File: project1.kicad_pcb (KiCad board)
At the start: 2 copper layers, 150.4 x 48.8 mm, 53 parts, among them P1 CONN_01X02, P10 CONN_02X01, P11 CONN_02X01, P12 CONN_02X01, P13 CONN_02X01, P14 CONN_02X01, P15 CONN_02X01, P16 CONN_02X01, P17 CONN_02X01, P18 CONN_02X01, P19 CONN_02X01, P2 CONN_01X04, P20 CONN_02X01, P21 CONN_02X01, P22 CONN_02X01, P23 CONN_02X01, P24 CONN_02X01, P25 CONN_02X01, P26 CONN_02X01, P27 CONN_02X01, P28 CONN_02X01, P29 CONN_02X01, P3 CONN_02X04, P4 CONN_02X04, P5 CONN_01X04, P6 CONN_02X04, P7 CONN_02X01, P8 CONN_02X01, P9 CONN_02X01, U1 LT1460GIZ-5, U2 TS912IN

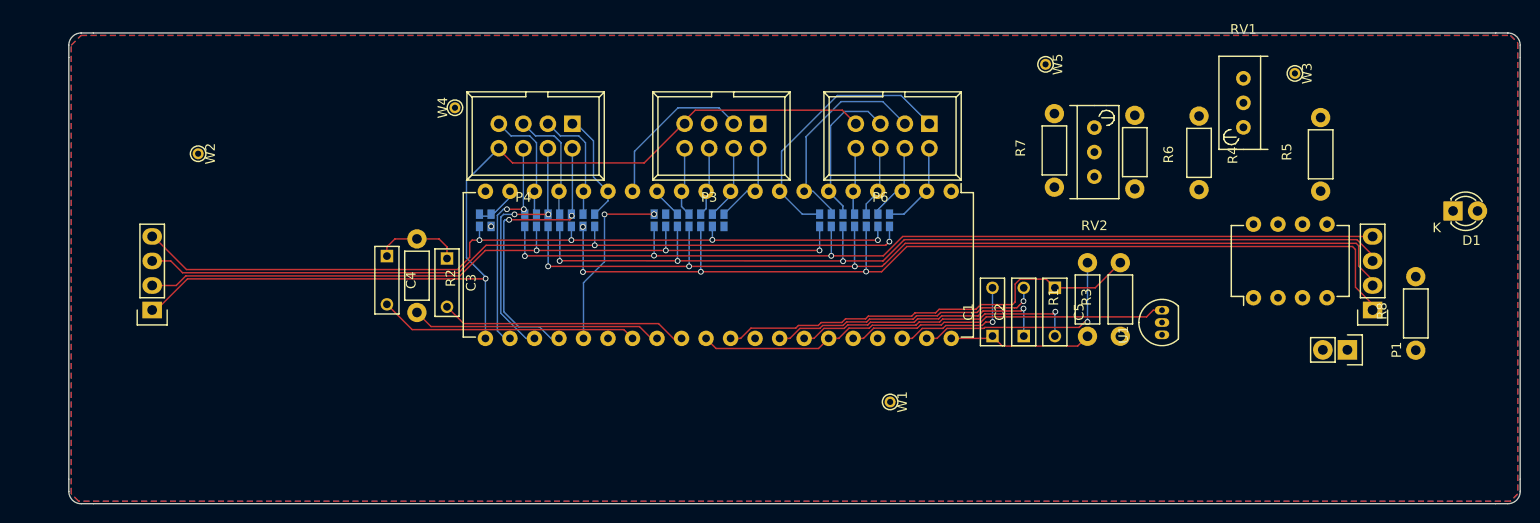
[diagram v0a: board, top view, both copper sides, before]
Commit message: latest revision
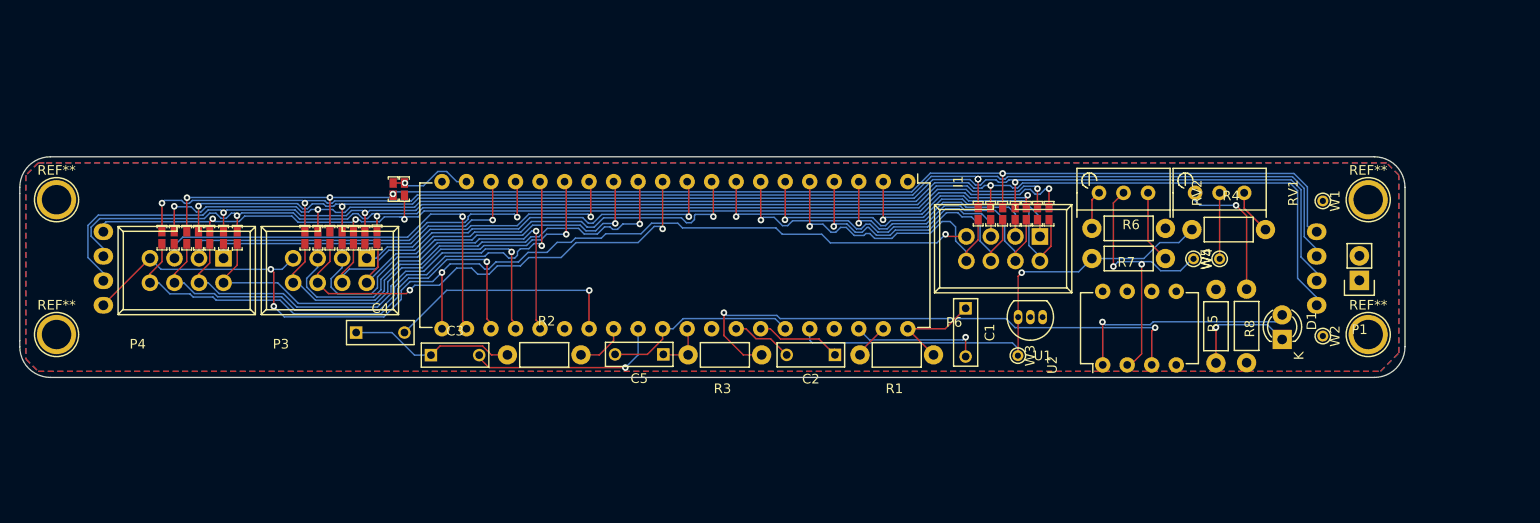
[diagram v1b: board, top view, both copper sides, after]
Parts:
- removed P2, P5: CONN_01X04, Pin_Headers:Pin_Header_Straight_1x04
- added LCD1: LCD-S101D40TR, IDC:LCD-S101D40TR, B.Cu at (135.0, 110.0)
- added REF**: 1pin, Connect:1pin, F.Cu at (67.3, 102.9)
- added REF**: 1pin, Connect:1pin, F.Cu at (203.2, 102.9)
- added REF**: 1pin, Connect:1pin, F.Cu at (203.2, 116.8)
- added REF**: 1pin, Connect:1pin, F.Cu at (67.3, 116.8)
- P10, P11, P12, P13, P14, P15, P16, P17, P18, P19, P20, P21, P22, P23, P24, P25, P26, P27, P28, P29, P7, P8, P9: moved to F.Cu
- moved W2 118.0 mm to (198.5, 117.0)
- moved W4 80.8 mm to (187.8, 109.0)
- moved W1 49.4 mm to (198.5, 103.0)
- moved P3 46.9 mm to (95.6, 110.2)
- moved P4 42.8 mm to (80.8, 110.2)
- moved C5 41.1 mm to (130.2, 118.9), turned to 180 degrees
- moved P24 41.1 mm to (80.8, 106.8)
- moved W3 41.0 mm to (166.9, 119.0)
- moved P23 40.0 mm to (78.2, 106.8)
- moved P15 39.8 mm to (93.0, 106.8)
- moved P16 38.5 mm to (95.6, 106.8)
- moved P25 37.5 mm to (83.2, 106.8)
- moved P28 37.5 mm to (82.0, 106.8)
- moved P17 37.2 mm to (98.1, 106.8)
- moved R3 37.2 mm to (140.4, 118.9), turned to 180 degrees
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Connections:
- P3 pad 1: G2 -> E2
- P3 pad 3: E2 -> F2
- P3 pad 5: F2 -> G2
- P4 pad 1: D3 -> E3
- P4 pad 2: C3 -> D3
- P4 pad 3: B3 -> F3
- P4 pad 4: A3 -> C3
- P4 pad 5: F3 -> G3
- P4 pad 6: G3 -> B3
- P4 pad 7: E3 -> BP
- P4 pad 8: BP -> A3
- P6 pad 3: G1 -> F1
- P6 pad 5: F1 -> G1
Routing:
- net Vin+: track 0.00 -> 56.4 mm, vias 0 -> 2
- net A2: track 7.56 -> 49.8 mm, vias 0 -> 1
- net G: track 98.2 -> 140.3 mm
- net B2: track 7.48 -> 49.2 mm, vias 0 -> 2
- net B3: track 12.7 -> 54.2 mm, vias 0 -> 1
- net F: track 97.3 -> 138.6 mm
- net Net-(C5-Pad1): track 45.5 -> 5.34 mm
- net C2: track 7.99 -> 48.0 mm, vias 0 -> 1
- net F2: track 3.93 -> 42.8 mm, vias 0 -> 1
- net D2: track 9.07 -> 47.9 mm, vias 0 -> 1
- net D3: track 12.0 -> 49.7 mm, vias 0 -> 1
- net E: track 78.2 -> 114.6 mm
- net A: track 102.2 -> 137.5 mm, vias 3 -> 4
- net B: track 103.0 -> 134.6 mm, vias 5 -> 4
- net D: track 81.8 -> 112.5 mm, vias 2 -> 3
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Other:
- board size 150.4 x 48.8 mm -> 143.5 x 22.9 mm
- net class Default: via_dia 0.6 -> 0.6858; via_drill 0.4 -> 0.3302
- rule via_min_drill: 0.3 -> 0.3302
- rule via_min_size: 0.4 -> 0.6858
